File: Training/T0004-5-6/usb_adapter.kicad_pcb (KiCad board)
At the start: 2 copper layers, 50.8 x 25.4 mm, 23 parts, among them J1 modular8_rev3_comms_out, P1 USB_OTG, U1 FT231X, U2 TE_1825058-1

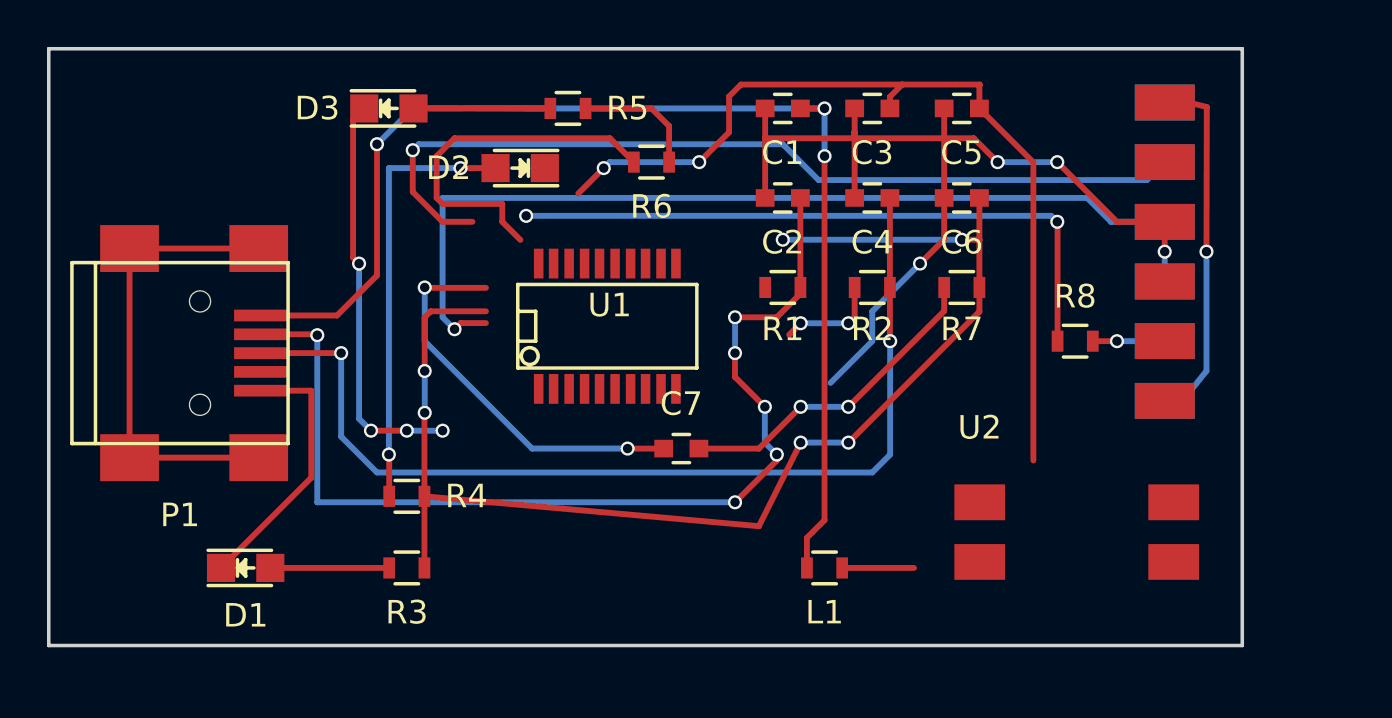
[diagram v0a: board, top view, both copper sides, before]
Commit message: finished routing after fix
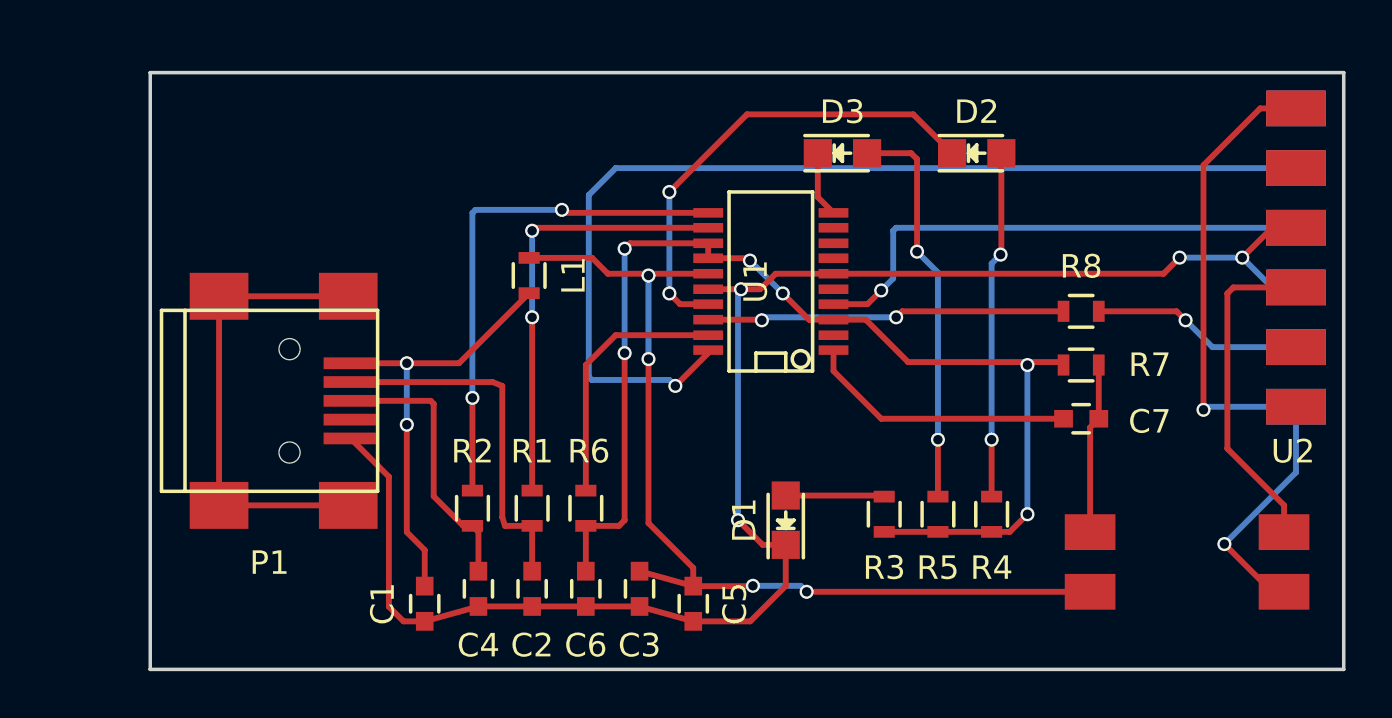
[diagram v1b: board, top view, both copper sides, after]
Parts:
- moved C1 26.0 mm to (153.9, 99.6), turned to 270 degrees
- moved R4 24.9 mm to (178.1, 95.8), turned to 90 degrees
- moved C5 24.0 mm to (165.4, 99.6), turned to 270 degrees
- moved C4 23.6 mm to (156.2, 98.9), turned to 270 degrees
- moved R5 23.4 mm to (175.8, 95.8), turned to 90 degrees
- moved C6 23.1 mm to (160.8, 98.9), turned to 270 degrees
- moved D1 23.1 mm to (169.3, 96.0), turned to 90 degrees
- moved C3 22.7 mm to (163.1, 98.9), turned to 270 degrees
- moved R3 20.4 mm to (173.5, 95.8), turned to 90 degrees
- moved C2 19.8 mm to (158.5, 98.9), turned to 270 degrees
- moved D2 19.4 mm to (177.4, 80.4), turned to 0 degrees
- moved R2 19.4 mm to (156.0, 95.5), turned to 270 degrees
- moved D3 19.4 mm to (171.7, 80.4)
- moved L1 17.7 mm to (158.4, 85.6), turned to 270 degrees
- moved C7 17.1 mm to (181.9, 91.7)
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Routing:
- net Net-(C1-Pad1): track 51.8 -> 18.6 mm, vias 3 -> 2
- net Net-(C4-Pad1): track 42.2 -> 11.7 mm, vias 2 -> 0
- net Net-(C2-Pad1): track 43.9 -> 15.5 mm, vias 6 -> 0
- net /~RXLED: track 0.06 -> 20.2 mm, vias 0 -> 2
- net Net-(R1-Pad1): track 0.00 -> 18.6 mm, vias 0 -> 2
- net Net-(R2-Pad1): track 4.36 -> 22.0 mm
- net /RX: track 38.4 -> 22.2 mm
- net GND: track 54.2 -> 68.8 mm
- net /~TXLED: track 17.3 -> 2.82 mm, vias 4 -> 0
- net /POWER_OUT: track 16.2 -> 29.8 mm, vias 1 -> 2
- net Net-(J1-Pad7): track 0.76 -> 14.2 mm
- net /TXDEN: track 27.8 -> 15.3 mm
- net Net-(D3-Pad2): track 5.84 -> 17.0 mm, vias 0 -> 2
- net +3V3: track 60.2 -> 49.4 mm
- net /PROGRAM: track 13.9 -> 7.26 mm, vias 2 -> 0
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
